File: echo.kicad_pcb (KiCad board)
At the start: 4 copper layers, 99.5 x 65 mm, 209 parts, among them J1 USB4215-03-A, J2 USB4215-03-A, J3 MDC-036, J4 DC3RX19JA2, J5 0475710001, J6 PJ-320D, J7 MDC-036, J8 SS-52100-004, Q1 BSS138, Q2 BSS138, Q3 AO3400A, Q4 AO3400A, Q5 BC850, Q6 BC850, Q7 AO3400A, Q8 AO3400A, U1 SN74CBT3257CDR, U10 AMS1117-3.3, U11 AMS1117-1.8, U12 RP2040, U13 W25Q128JVSIQ, U14 MW7211A, U15 TS3USB221RSER, U2 CH340C, U3 USBLC6-2SC6, U4 USBLC6-2SC6, U5 NCP1117 3.3, U6 W25Q32JVSIQ, U7 ESP32-D0WD, U8 ESP-PSRAM32, U9 MS9288A, X1 24.576 MHz, Y1 40 MHz, Y2 12 MHz

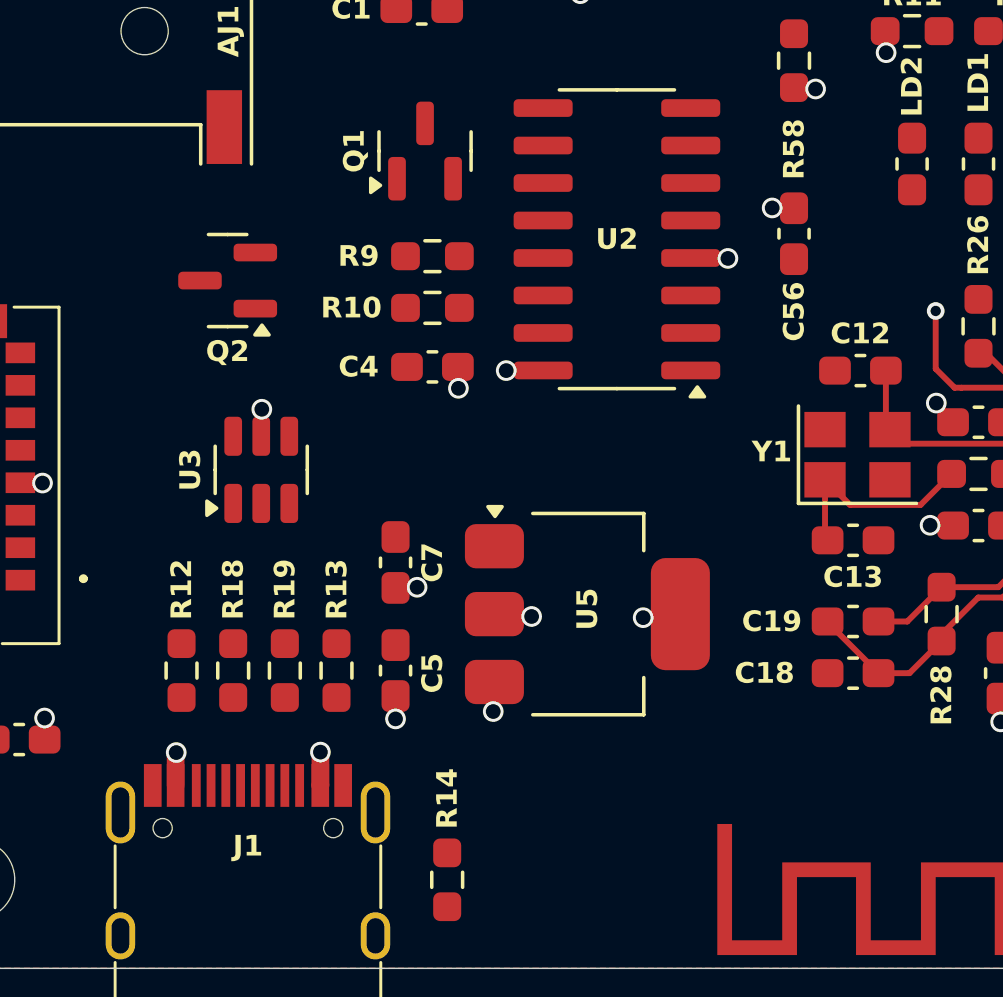
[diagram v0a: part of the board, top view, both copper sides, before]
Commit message: Update echo.kicad_pcb
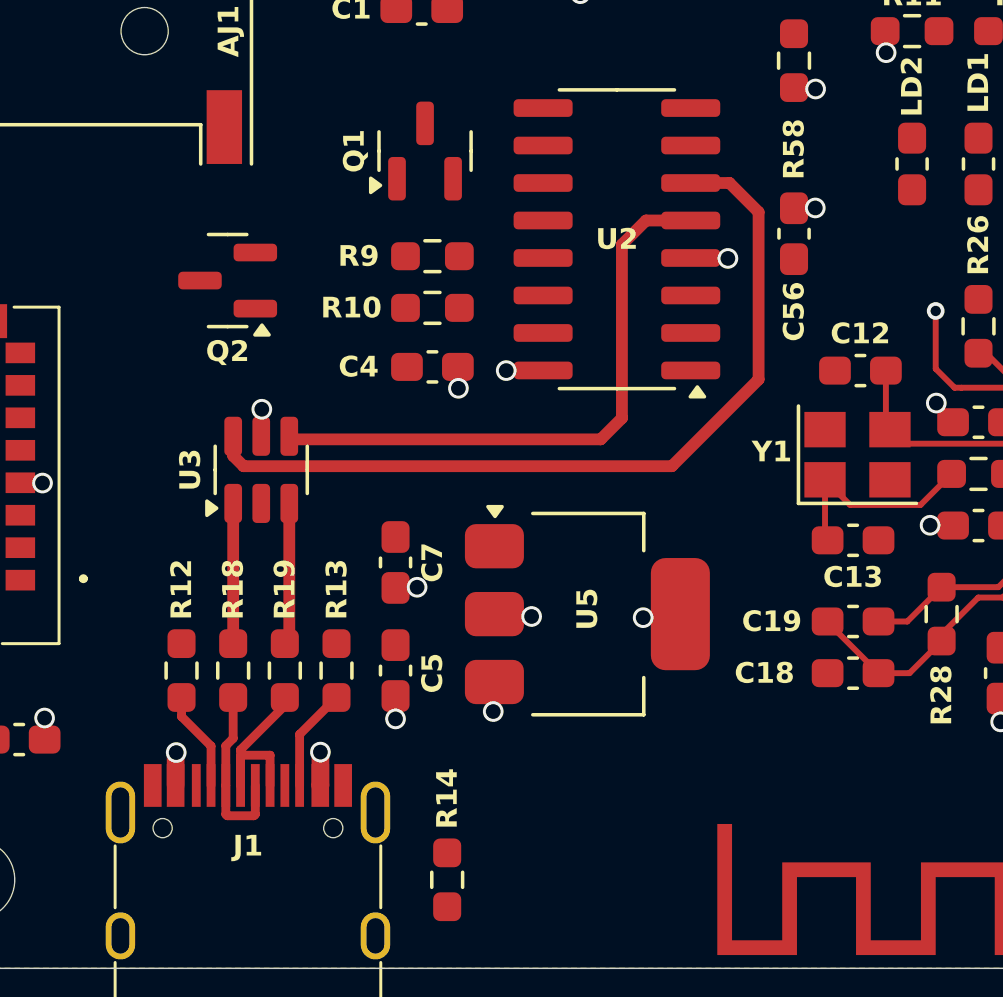
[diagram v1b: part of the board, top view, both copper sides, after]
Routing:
- net /TC1_D-: track 0.00 -> 28.2 mm
- net /TC1_D+: track 0.00 -> 20.2 mm
- net Net-(J1-DP1): track 0.00 -> 6.62 mm
- net Net-(J1-DN1): track 0.00 -> 6.08 mm
- net Net-(R19-Pad1): track 0.00 -> 4.81 mm
- net Net-(R18-Pad1): track 0.00 -> 4.75 mm
- net Net-(J1-CC2): track 0.00 -> 3.50 mm
- net Net-(J1-CC1): track 0.00 -> 3.39 mm

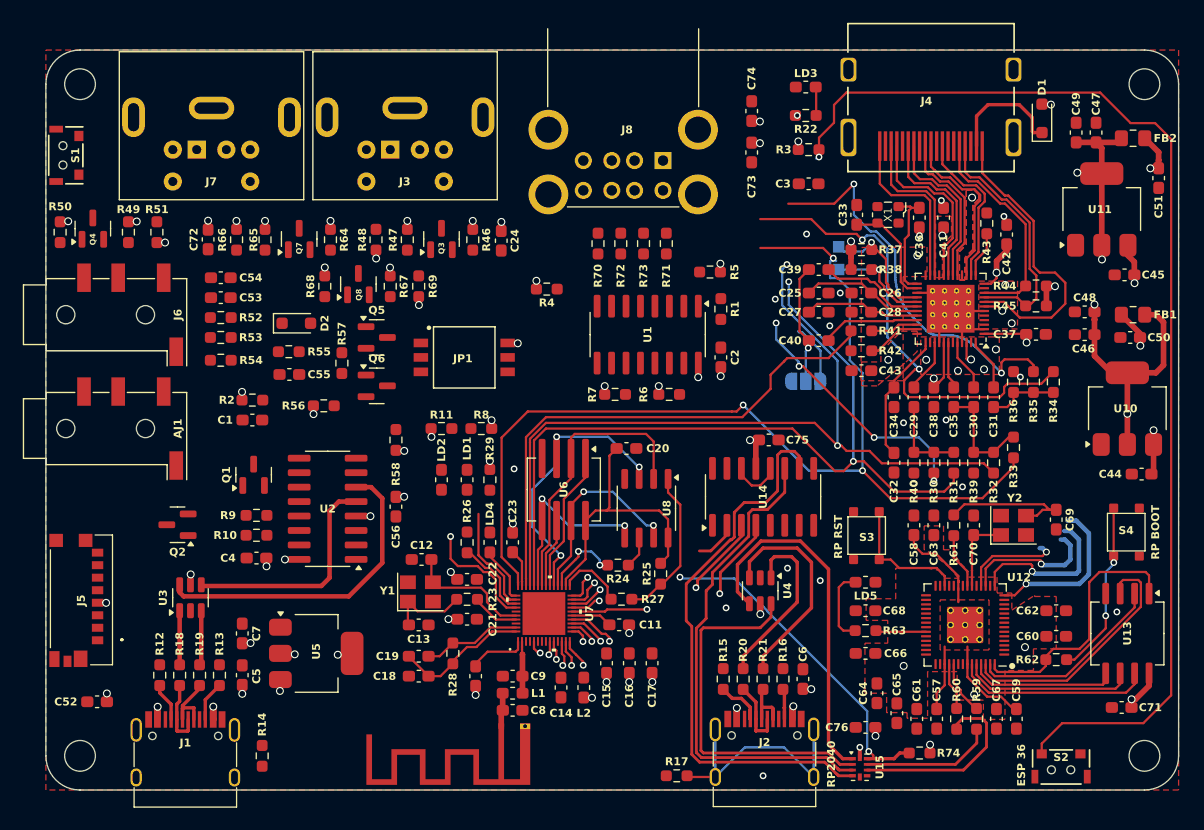
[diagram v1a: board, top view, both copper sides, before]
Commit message: 1.06 WIP
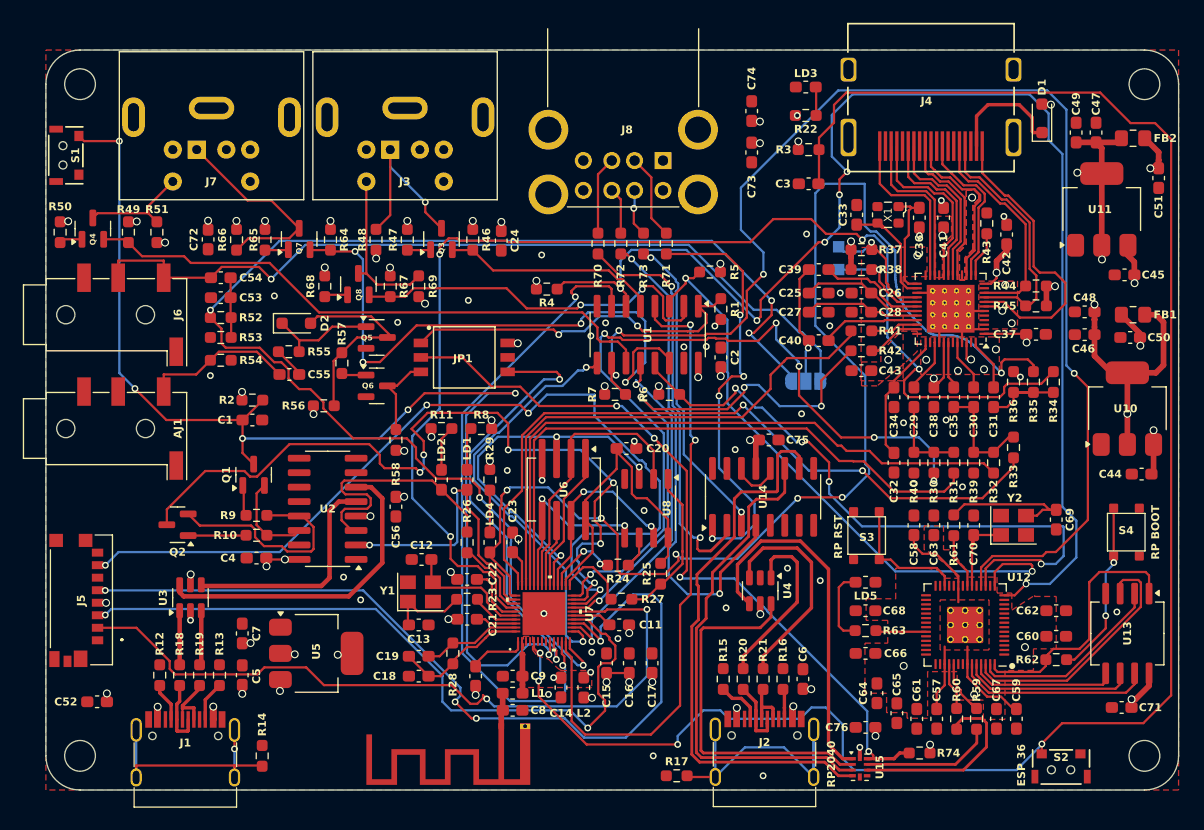
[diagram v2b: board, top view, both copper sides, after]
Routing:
- net /ESP_IO25: track 2.61 -> 117.7 mm, vias 1 -> 5
- net /GPIO15: track 8.79 -> 114.9 mm, vias 1 -> 4
- net /ESP_EN: track 1.20 -> 105.3 mm, vias 1 -> 6
- net /GPIO11: track 14.2 -> 115.6 mm, vias 1 -> 6
- net /ESP_IO2: track 3.00 -> 80.9 mm, vias 2 -> 4
- net /ESP_IO14: track 3.22 -> 76.9 mm, vias 1 -> 4
- net /ESP_IO22: track 39.4 -> 111.0 mm, vias 2 -> 6
- net /A_OUT: track 5.37 -> 73.3 mm, vias 0 -> 1
- net /ESP_IO0: track 2.96 -> 69.8 mm, vias 1 -> 6
- net /ESP_IO13: track 6.68 -> 66.5 mm, vias 1 -> 2
- net /ESP_IO36: track 100.7 -> 160.4 mm, vias 2 -> 4
- net /ESP_IO12: track 4.28 -> 62.4 mm, vias 1 -> 2
- net /ESP_IO21: track 52.0 -> 109.3 mm, vias 3 -> 4
- net /ESP_IO32: track 2.25 -> 57.2 mm, vias 1 -> 2
- net /ESP_IO33: track 2.32 -> 57.0 mm, vias 1 -> 2
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- added copper zone on F.Cu, net +3.3VP
- added copper zone on In2.Cu, net +3.3VP
